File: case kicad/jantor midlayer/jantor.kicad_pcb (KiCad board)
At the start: 2 copper layers, 165.5 x 99.1 mm, 0 parts

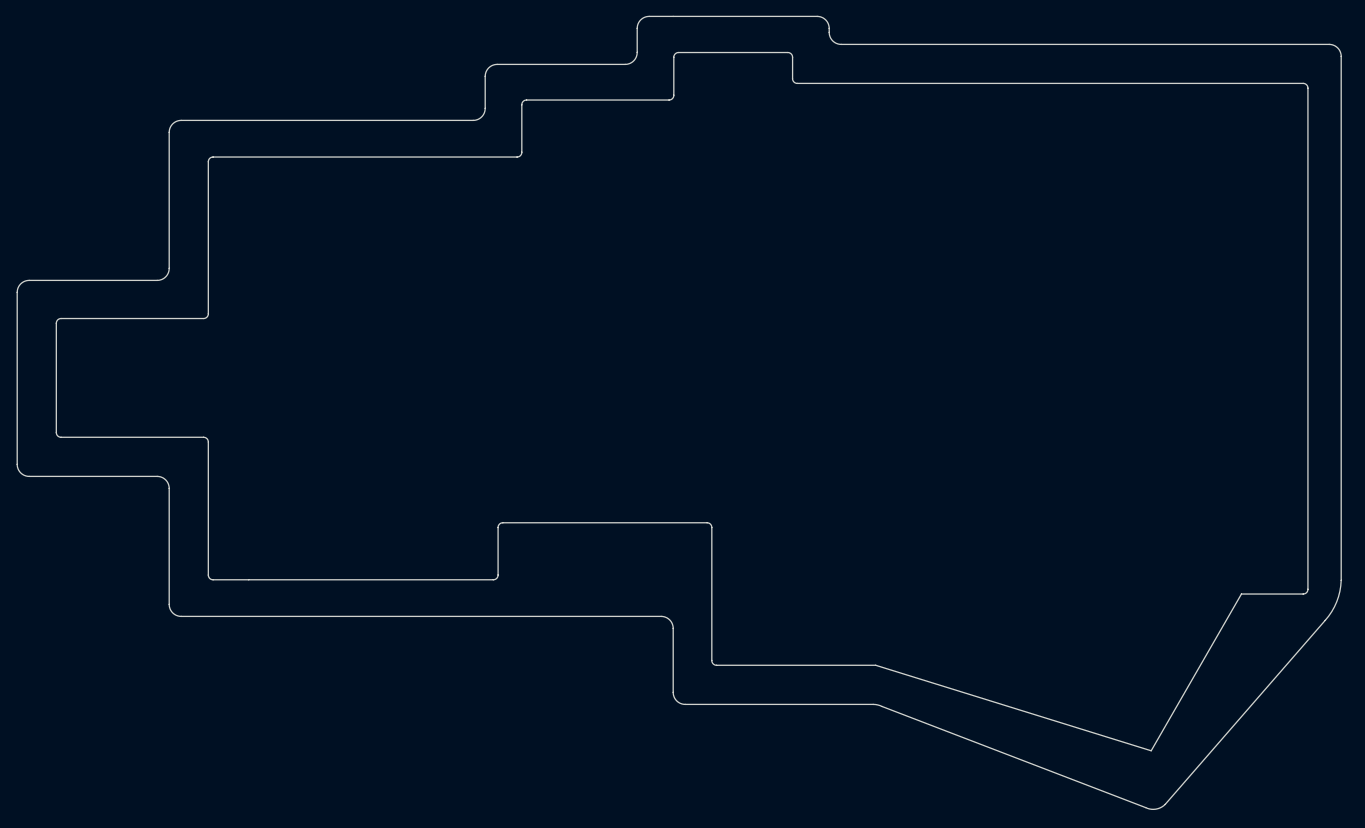
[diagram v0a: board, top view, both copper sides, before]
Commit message: hehehe i dont remember ANYTHING
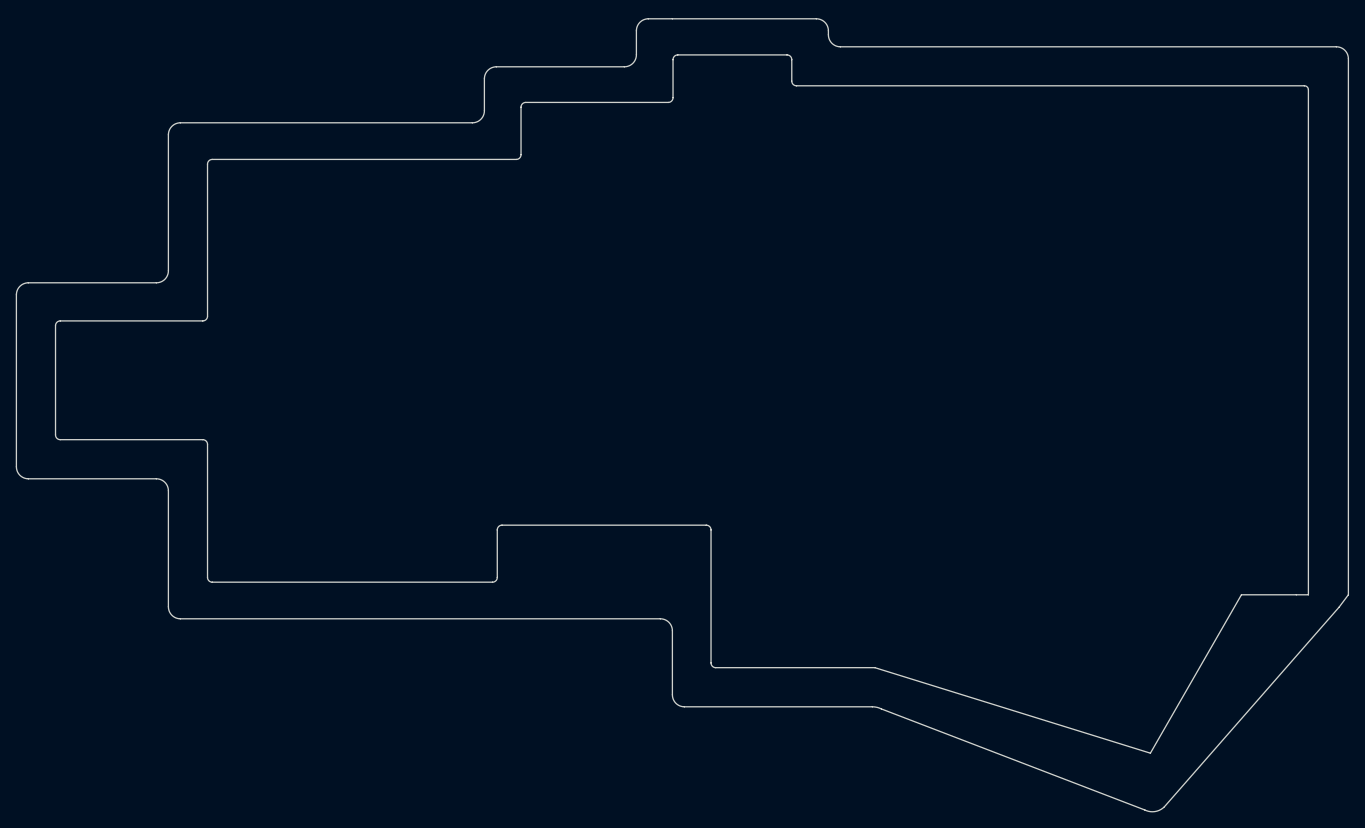
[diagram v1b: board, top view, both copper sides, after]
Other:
- board size 165.5 x 99.1 mm -> 166.5 x 99.1 mm
